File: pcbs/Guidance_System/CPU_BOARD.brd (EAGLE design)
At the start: 100 x 52.1 mm, 33 parts, among them J1 22-27-2081-08, J10 22-27-2081-08, J11 22-27-2081-08, J12 22-27-2081-08, J13 22-27-2081-08, J14 22-27-2081-08, J15 22-27-2041-04, J16 22-27-2041-04, J17 22-27-2021-02, J2 22-27-2021-02, J3 22-27-2041-04, J4 22-27-2041-04, J5 22-27-2081-08, J6 22-27-2021-02, J7 22-27-2081-08, J8 22-27-2021-02, J9 22-27-2021-02

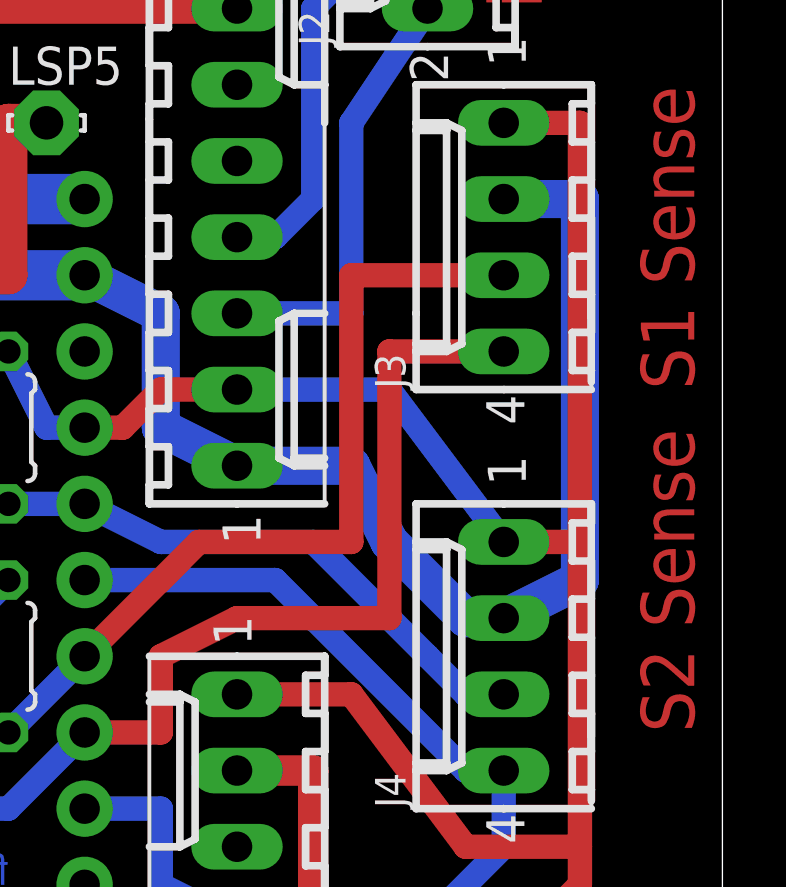
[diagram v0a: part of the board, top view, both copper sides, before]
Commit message: * Fixed Track
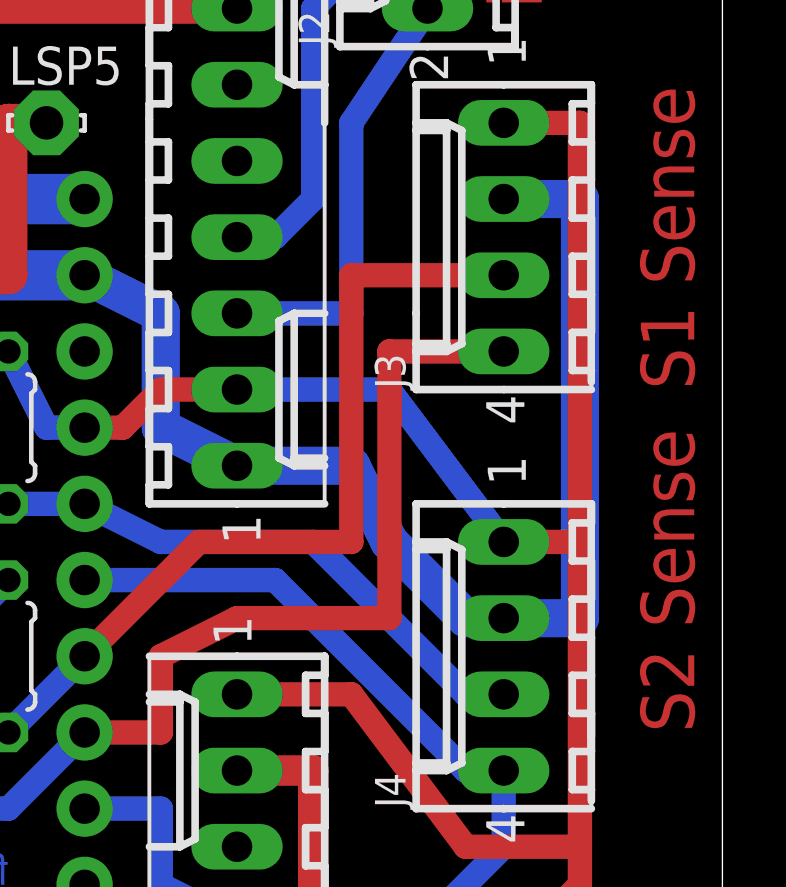
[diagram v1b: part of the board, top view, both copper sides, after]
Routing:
- net N$24: track 59.4 -> 60.4 mm
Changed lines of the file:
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@@
 <grid distance="0.05" unitdist="inch" unit="inch" style="lines" multiple="1" display="no" altdistance="0.025" altunitdist="inch" altunit="inch"/>
 <layers>
-<layer number="1" name="Top" color="4" fill="1" visible="yes" active="yes"/>
-<layer number="16" name="Bottom" color="1" fill="1" visible="no" active="yes"/>
+<layer number="1" name="Top" color="4" fill="1" visible="no" active="yes"/>
+<layer number="16" name="Bottom" color="1" fill="1" visible="yes" active="yes"/>
 <layer number="17" name="Pads" color="2" fill="1" visible="yes" active="yes"/>
 <layer number="18" name="Vias" color="2" fill="1" visible="yes" active="yes"/>
@@
 <contactref element="R3" pad="1"/>
 <wire x1="92.71" y1="49.53" x2="91.44" y2="49.53" width="0.8128" layer="16"/>
-<wire x1="91.44" y1="49.53" x2="90.17" y2="50.8" width="0.8128" layer="16"/>
-<wire x1="90.17" y1="50.8" x2="86.36" y2="54.61" width="0.8128" layer="16"/>
+<wire x1="91.44" y1="49.53" x2="86.36" y2="54.61" width="0.8128" layer="16"/>
 <wire x1="86.36" y1="54.61" x2="81.28" y2="54.61" width="0.8128" layer="16"/>
 <wire x1="81.28" y1="54.61" x2="78.74" y2="55.88" width="0.8128" layer="16"/>
@@
 <contactref element="J3" pad="2"/>
 <wire x1="92.71" y1="66.04" x2="95.25" y2="66.04" width="1.27" layer="16"/>
-<wire x1="95.25" y1="66.04" x2="95.25" y2="53.34" width="1.27" layer="16"/>
-<wire x1="95.25" y1="53.34" x2="92.71" y2="52.07" width="1.27" layer="16"/>
+<wire x1="95.25" y1="66.04" x2="95.25" y2="52.07" width="1.27" layer="16"/>
+<wire x1="95.25" y1="52.07" x2="92.71" y2="52.07" width="1.27" layer="16"/>
 <wire x1="92.71" y1="52.07" x2="91.44" y2="52.07" width="1.27" layer="16"/>
 <wire x1="91.44" y1="52.07" x2="88.9" y2="54.61" width="1.27" layer="16"/>
